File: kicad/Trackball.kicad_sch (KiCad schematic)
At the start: 47 parts, among them J1 Conn_01x04, J10 Conn_01x01_Female, J3 Conn_02x03_Odd_Even, J4 Conn_01x06_Pin, J7 Conn_01x01_Female, SW1 Push_Button, SW2 Push_Button, SW3 RotaryEncoder, SW4 Push_Button, U1 TCR2EF19, U2 PMW3360, U3 TLV73333PDBV, U4 ESP32-S3-WROOM-1, U5 TP4056, U6 DW01, U7 FS8205A

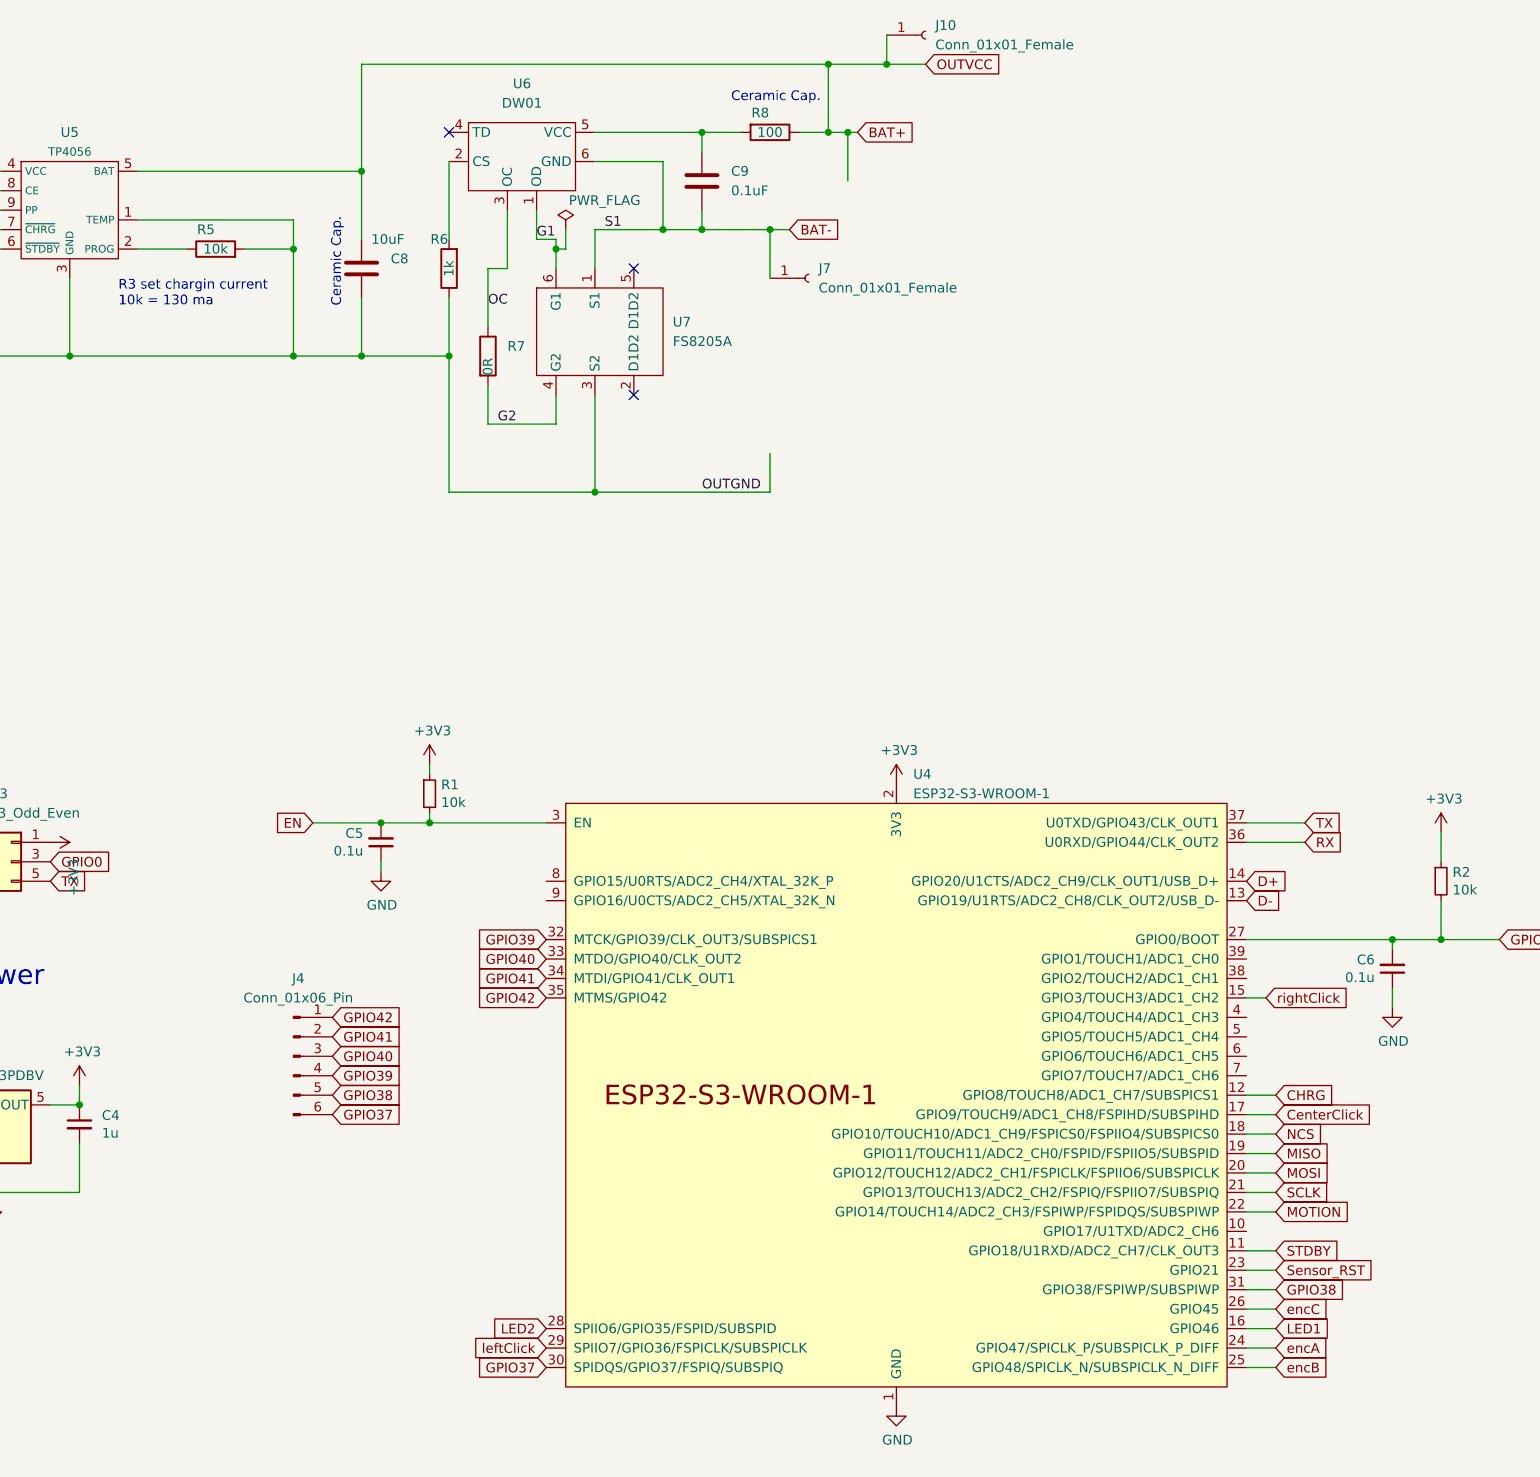
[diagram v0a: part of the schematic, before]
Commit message: next routing try
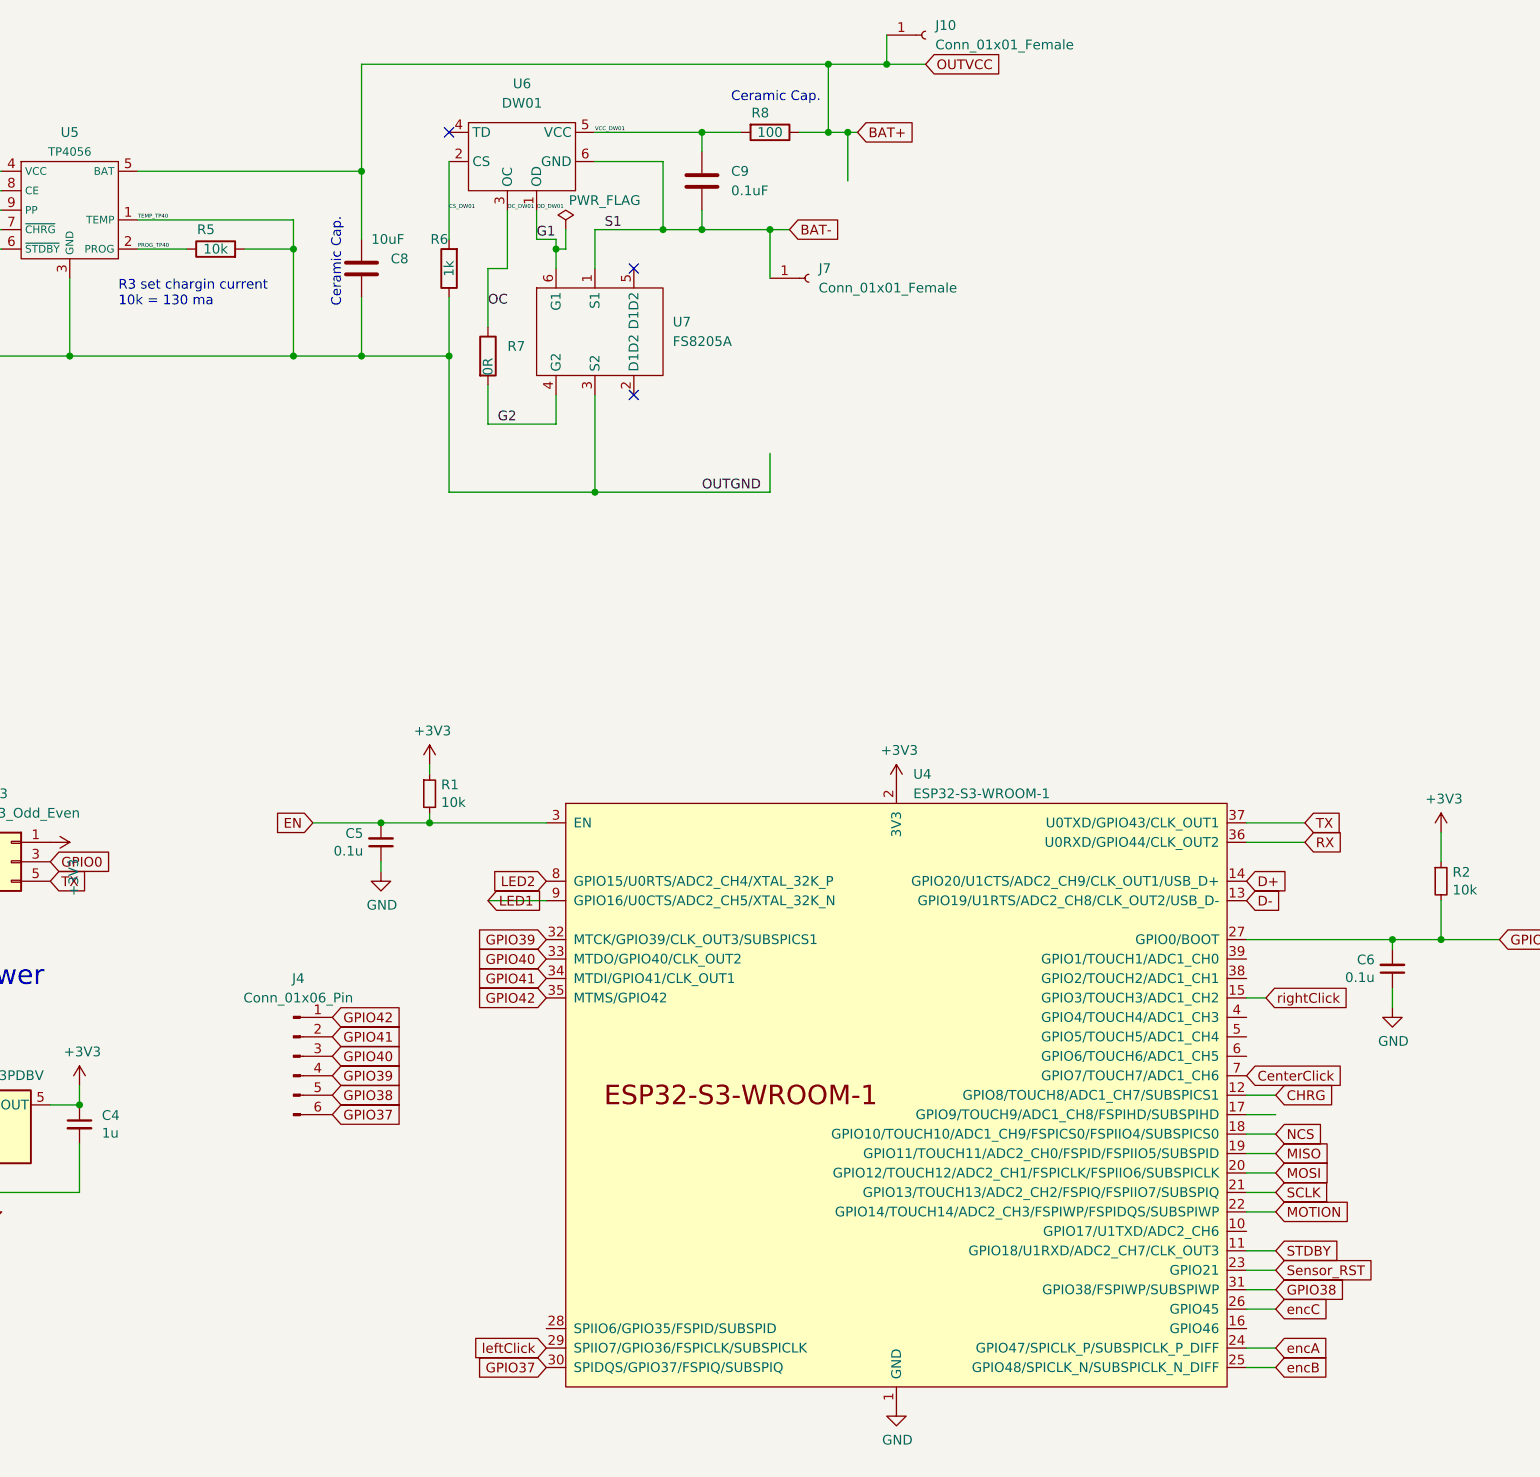
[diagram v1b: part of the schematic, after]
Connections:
- net CenterClick: now also U4.7 (GPIO7/TOUCH7/ADC1_CH6); no longer U4.17 (GPIO9/TOUCH9/ADC1_CH8/FSPIHD/SUBSPIHD)
- net LED1: now also U4.9 (GPIO16/U0CTS/ADC2_CH5/XTAL_32K_N); no longer U4.16 (GPIO46)
- net LED2: now also U4.8 (GPIO15/U0RTS/ADC2_CH4/XTAL_32K_P); no longer U4.28 (SPIIO6/GPIO35/FSPID/SUBSPID)
- net PROG_TP40: now reaches R5.1, U5.2 (PROG)
- net VCC_DW01: now reaches C9.1, R8.2, U6.5 (VCC)
- net CS_DW01: now reaches R6.2, U6.2 (CS)
